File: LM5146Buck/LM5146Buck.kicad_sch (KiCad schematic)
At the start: 7 parts

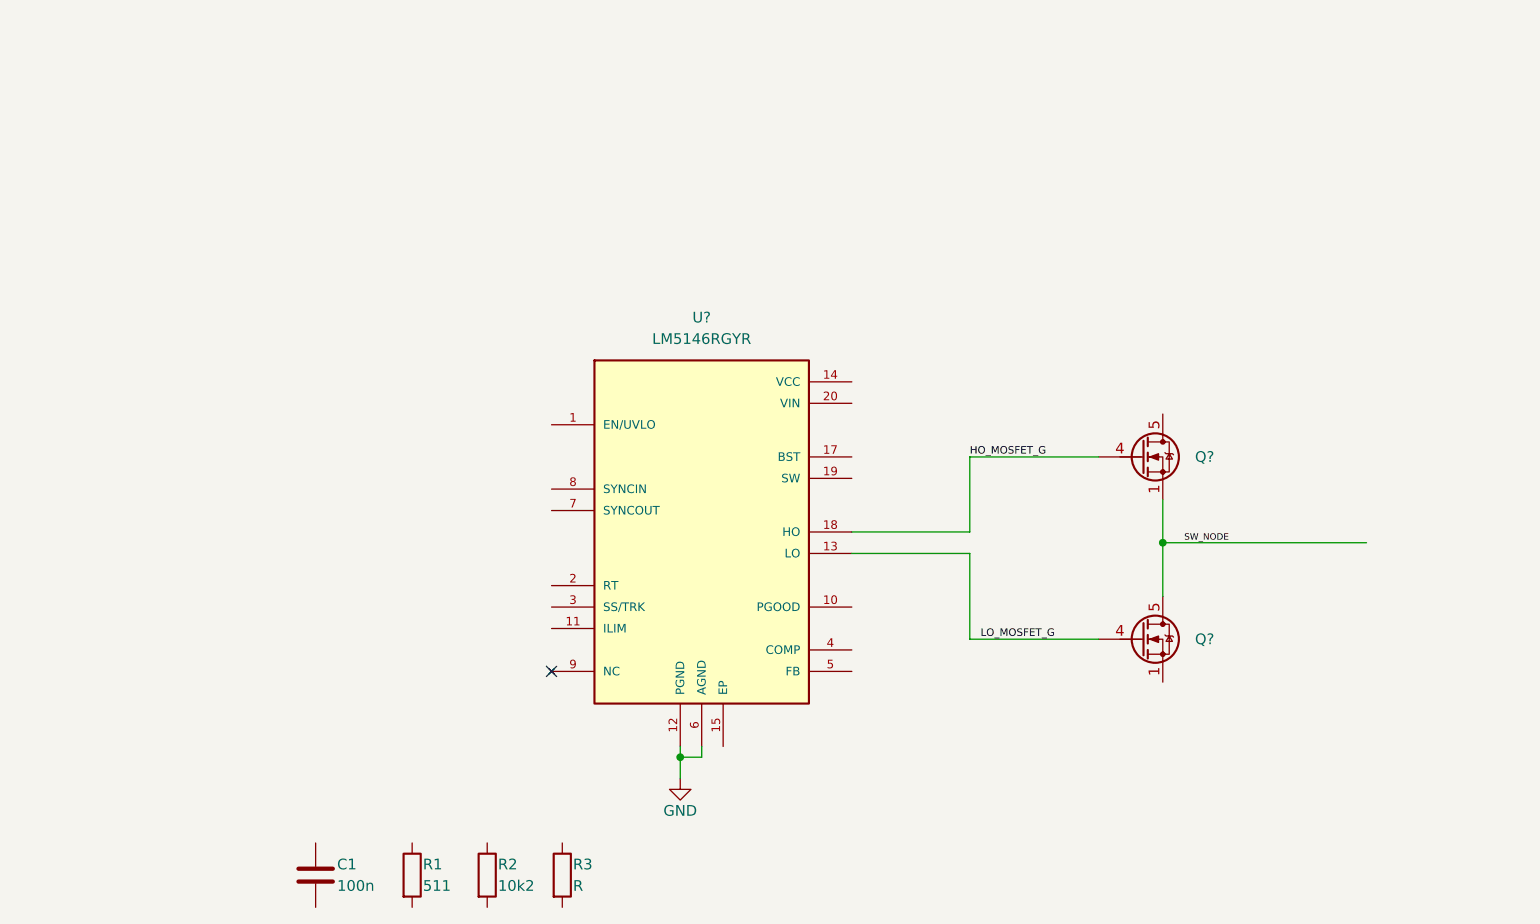
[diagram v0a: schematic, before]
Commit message: Update LM5146Buck.kicad_sch
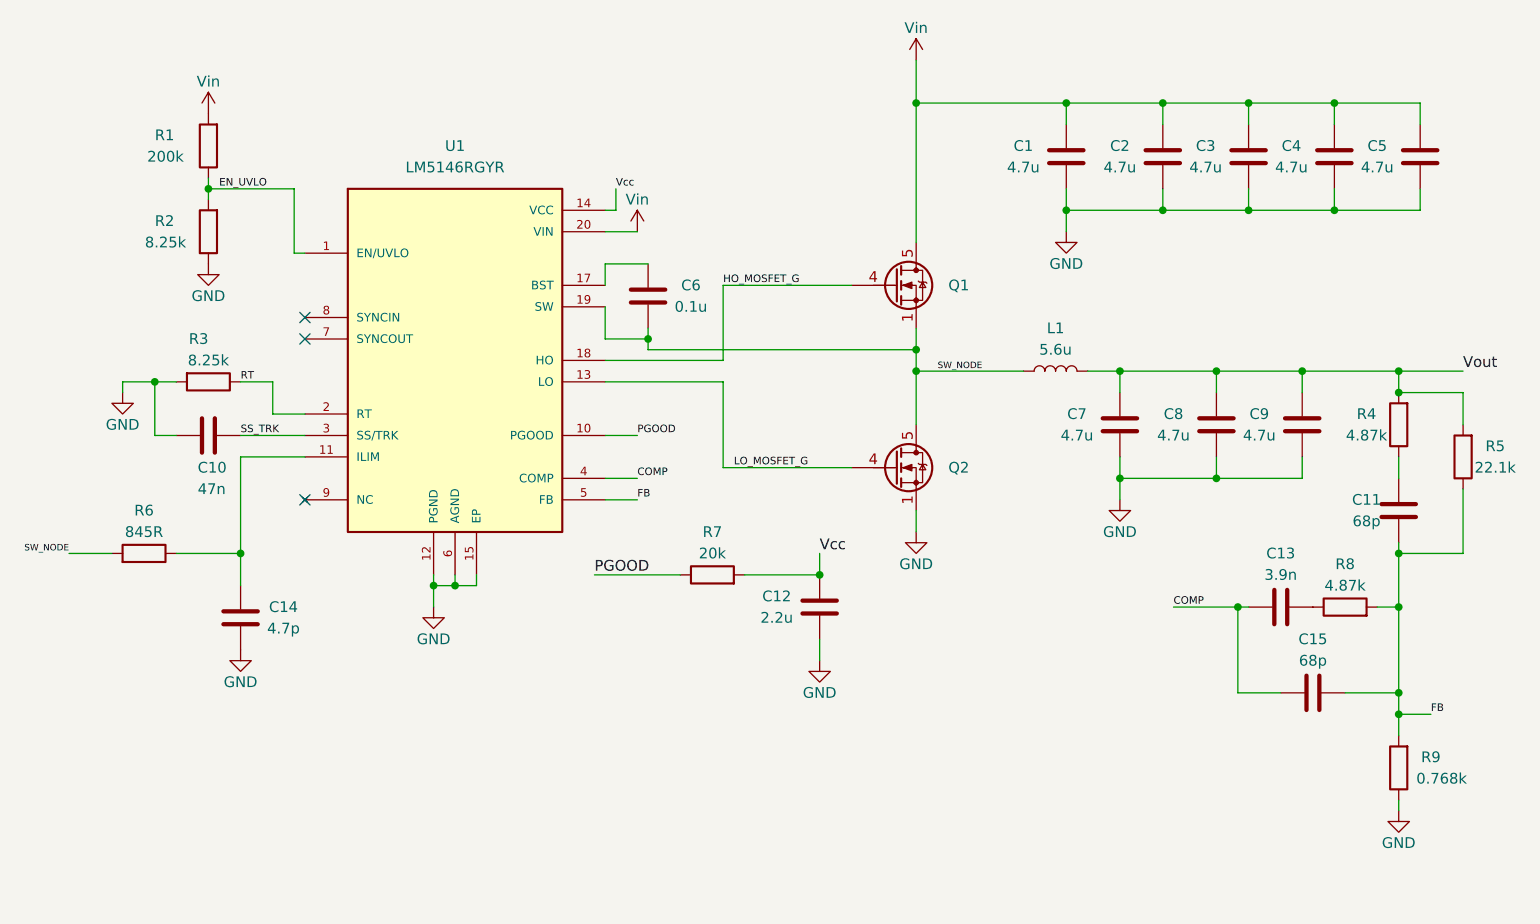
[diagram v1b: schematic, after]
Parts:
- added C1, C2, C3, C4, C5, C7, C8, C9: 4.7u, Capacitor_SMD:C_0603_1608Metric, symbol Device:C
- added C11, C15: 68p, Capacitor_SMD:C_0603_1608Metric, symbol Device:C
- added C12: 2.2u, Capacitor_SMD:C_0603_1608Metric, symbol Device:C
- added C13: 3.9n, Capacitor_SMD:C_0603_1608Metric, symbol Device:C
- added C14: 4.7p, Capacitor_SMD:C_0603_1608Metric, symbol Device:C
- added C6: 0.1u, Capacitor_SMD:C_0603_1608Metric, symbol Device:C
- added L1: 5.6u, symbol Device:L
- added R1: 200k, Resistor_SMD:R_0603_1608Metric, symbol Device:R
- added R4: 4.87k, Resistor_SMD:R_0603_1608Metric, symbol Device:R
- added R5: 22.1k, Resistor_SMD:R_0603_1608Metric, symbol Device:R
- added R6: 845R, Resistor_SMD:R_0603_1608Metric, symbol Device:R
- added R7: 20k, Resistor_SMD:R_0603_1608Metric, symbol Device:R
- added R9: 0.768k, Resistor_SMD:R_0603_1608Metric, symbol Device:R
- C10: renamed from C1; value 100n -> 47n
- R2: renamed from R1; value 511 -> 8.25k
- R3: value R -> 8.25k
- R8: renamed from R2; value 10k2 -> 4.87k
- gave numbers to parts that had none: 3
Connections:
- net GND is gone; now on net EP: U1.12 (PGND), U1.6 (AGND)
- net EP: now also C10.2, Q2.1 (S), Q2.2 (S), Q2.3 (S), R2.1, R3.2, C1.1, C12.1, C14.1, C2.1, C3.1, C4.1, C5.1, C7.1, C8.1, C9.1, R9.1
- net SW_NODE: now also U1.19 (SW), C6.1, L1.1, R6.2
- net at R8.1: now also C13.2
- net FB: now reaches R8.2
- net FB: now also U1.5 (FB), C11.1, C15.2, R5.1, R9.2
- net SS_TRK: now reaches C10.1
- net SS_TRK: now also U1.3 (SS/TRK)
- net EN_UVLO: now reaches U1.1 (EN/UVLO)
- net EN_UVLO: now also R2.2, R1.1
- net PGOOD: now reaches U1.10 (PGOOD)
- net PGOOD: now also R7.1
- net at U1.11 (ILIM): now also C14.2, R6.1
- net Vcc: now reaches U1.14 (VCC)
- net Vcc: now also C12.2, R7.2
- net at U1.17 (BST): now also C6.2
- net RT: now reaches U1.2 (RT)
- net RT: now also R3.1
- net Vin: now reaches U1.20 (VIN)
- net Vin: now also Q1.5 (D), C1.2, C2.2, C3.2, C4.2, C5.2, R1.2
- net COMP: now reaches U1.4 (COMP)
- net COMP: now also C13.1, C15.1
- new net: C11.2, R4.1
- new net Vout: C7.2, C8.2, C9.2, L1.2, R4.2, R5.2
- no-connect marks 1 -> 3
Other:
- moved on the sheet: C10, Q1, Q2, R2, R8, U1
